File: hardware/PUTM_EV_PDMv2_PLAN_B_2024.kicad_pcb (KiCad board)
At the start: 4 copper layers, 58 x 87.3 mm, 22 parts, among them J2 74650073R, J5 UMPT-08-01-L-RA-WT-P-TR, J8 UMPT-08-01-L-RA-WT-P-TR

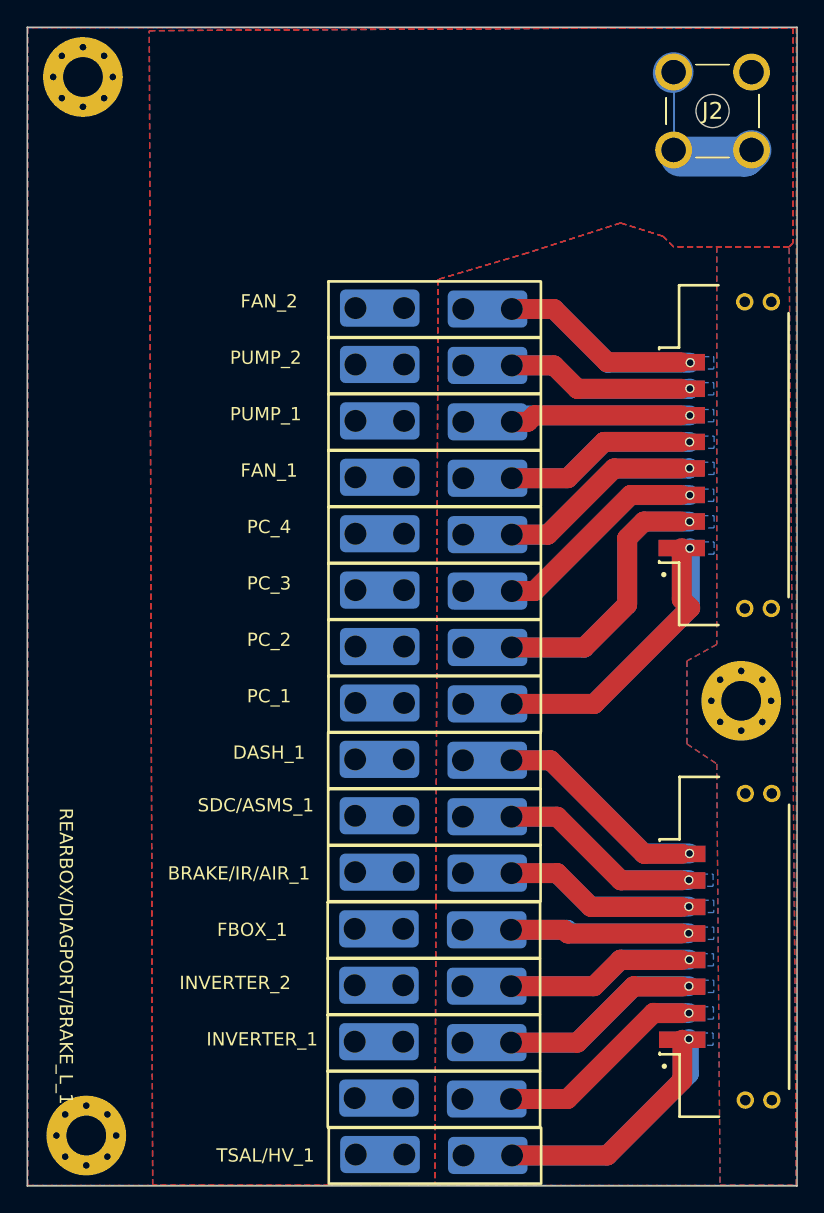
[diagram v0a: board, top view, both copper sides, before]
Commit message: Version_after_fix
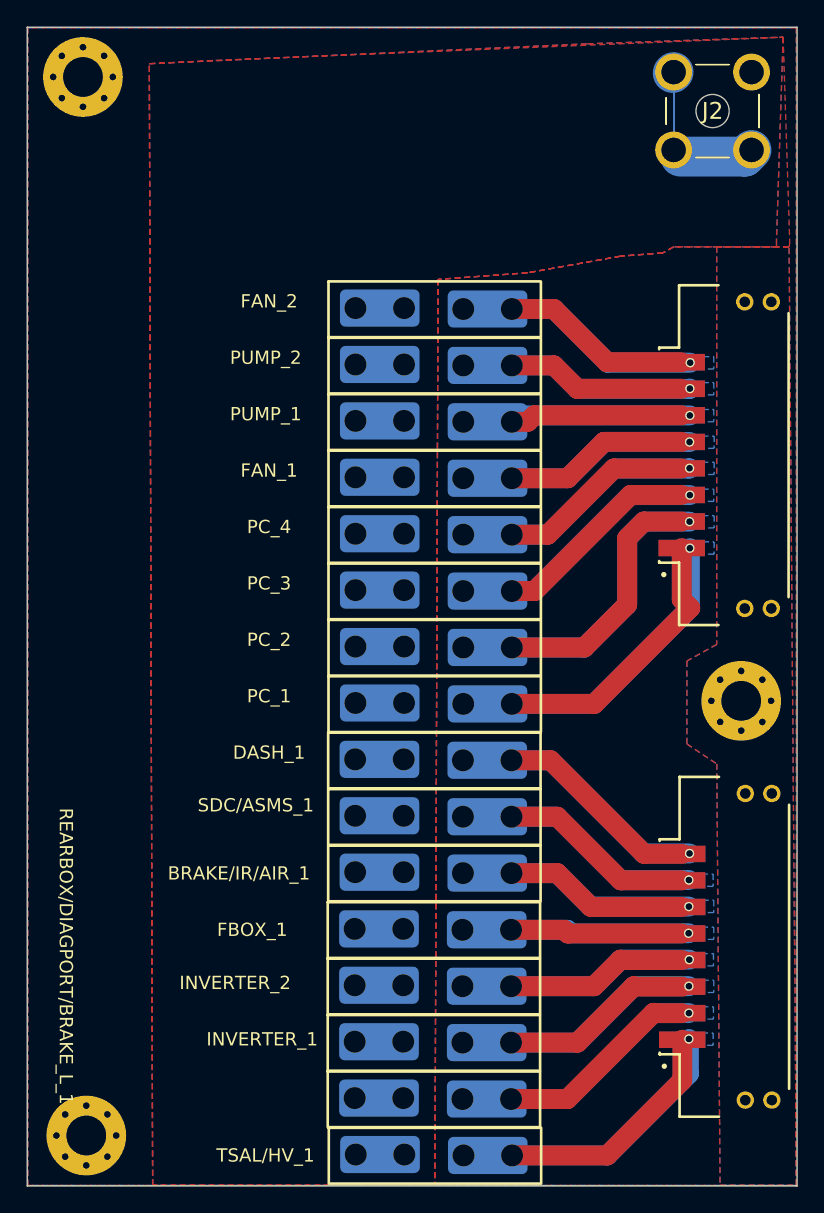
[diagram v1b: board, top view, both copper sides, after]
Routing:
- removed copper zone on In1.Cu, net GND
- removed copper zone on In2.Cu, net GND
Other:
- copper layers 4 -> 2
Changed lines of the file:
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@@
 	(layers
 		(0 "F.Cu" signal)
-		(4 "In1.Cu" signal)
-		(6 "In2.Cu" signal)
 		(2 "B.Cu" signal)
 		(13 "F.Paste" user)
@@
 			)
 			(layer "dielectric 1"
-				(type "prepreg")
+				(type "core")
 				(color "#505543FF")
-				(thickness 0.1)
-				(material "FR4")
-				(epsilon_r 4.5)
-				(loss_tangent 0.02)
-			)
-			(layer "In1.Cu"
-				(type "copper")
-				(thickness 0.0175)
-			)
-			(layer "dielectric 2"
-				(type "prepreg")
-				(color "#505543FF")
-				(thickness 1.24)
-				(material "FR4")
-				(epsilon_r 4.5)
-				(loss_tangent 0.02)
-			)
-			(layer "In2.Cu"
-				(type "copper")
-				(thickness 0.0175)
-			)
-			(layer "dielectric 3"
-				(type "prepreg")
-				(color "#505543FF")
-				(thickness 0.1)
+				(thickness 1.475)
 				(material "FR4")
 				(epsilon_r 4.5)
@@
 		(polygon
 			(pts
-				(xy 178.5 70.75) (xy 178.2 71.05) (xy 169.5 71.05) (xy 168.7 70.25) (xy 165.5 69.25) (xy 158.5 71.5)
-				(xy 151.75 73.5) (xy 151.52 141.75) (xy 130.25 141.75) (xy 130 54.76262) (xy 167.5 54.55) (xy 178.5 54.55)
+				(xy 178.25 70.75) (xy 178.2 71.05) (xy 169.5 71.05) (xy 168.7 71.5) (xy 165.5 71.75) (xy 158.5 73)
+				(xy 151.75 73.5) (xy 151.52 141.75) (xy 130.25 141.75) (xy 130 57.25) (xy 135 57) (xy 177.75 55.25)
 			)
 		)
@@
 		(polygon
 			(pts
-				(xy 178.5 70.75) (xy 178.2 71.05) (xy 169.5 71.05) (xy 168.7 70.25) (xy 165.5 69.25) (xy 158.5 71.5)
-				(xy 151.75 73.5) (xy 151.52 141.75) (xy 130.25 141.75) (xy 130 54.76262) (xy 167.5 54.55) (xy 178.5 54.55)
+				(xy 177.25 70.5) (xy 177.25 71.05) (xy 169.5 71.05) (xy 168.7 71.5) (xy 165.5 71.75) (xy 158.5 73)
+				(xy 151.75 73.5) (xy 151.52 141.75) (xy 130.25 141.75) (xy 130 57.25) (xy 163 55.75) (xy 177.75 55.25)
 			)
 		)
@@
 		(net 0)
 		(net_name "")
-		(layer "F.Mask")
-		(hatch edge 0.5)
-		(priority 2)
-		(connect_pads yes
-			(clearance 0.2)
-		)
-		(min_thickness 0)
-		(filled_areas_thickness no)
-		(fill yes
-			(thermal_gap 0.5)
-			(thermal_bridge_width 0.5)
-		)
-		(polygon
-			(pts
-				(xy 168.4 131.36) (xy 168.4 133.22) (xy 170.055 133.22) (xy 171.9 131.375) (xy 171.9 131.36)
-			)
-		)
-	)
-	(zone
-		(net 0)
-		(net_name "")
 		(layer "B.Cu")
 		(hatch edge 0.5)
@@
 		(hatch edge 0.5)
 		(connect_pads yes
-			(clearance 0.7)
+			(clearance 0.3)
 		)
 		(min_thickness 0.2)
@@
 			)
 		)
-	)
-	(zone
-		(net 1)
-		(net_name "GND")
-		(layer "In1.Cu")
-		(hatch edge 0.5)
-		(priority 1)
-		(connect_pads yes
-			(clearance 0.2)
-		)
-		(min_thickness 0.2)
-		(filled_areas_thickness no)
-		(fill yes
-			(thermal_gap 0.25)
-			(thermal_bridge_width 0.5)
-			(smoothing fillet)
-			(radius 0.25)
-		)
-		(polygon
-			(pts
-				(xy 120.85 54.55) (xy 120.85 141.75) (xy 178.75 141.75) (xy 178.75 54.55)
-			)
-		)
-	)
-	(zone
-		(net 1)
-		(net_name "GND")
-		(layer "In2.Cu")
-		(hatch edge 0.5)
-		(priority 1)
-		(connect_pads yes
-			(clearance 0.2)
-		)
-		(min_thickness 0.2)
-		(filled_areas_thickness no)
-		(fill yes
-			(thermal_gap 0.25)
-			(thermal_bridge_width 0.5)
-			(smoothing fillet)
-			(radius 0.25)
-		)
-		(polygon
-			(pts
-				(xy 120.85 54.55) (xy 120.85 141.75) (xy 178.75 141.75) (xy 178.75 54.55)
-			)
-		)

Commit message: Version_after_fix2
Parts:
- FAN_1, FAN_2, FBOX_1, INVERTER_1, INVERTER_2, PC_2, PC_3, PC_4, PUMP_1, PUMP_2, SDC/ASMS_1: value ~ -> 2A
- PC_1: value 1 -> 2A
